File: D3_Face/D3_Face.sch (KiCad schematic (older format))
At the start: 31 parts, among them J1 Conn_01x05_Male, U1 MAX7219, U2 MAX7219, U3 MAX7219, U4 MAX7219, U5 MAX7219, U6 MAX7219

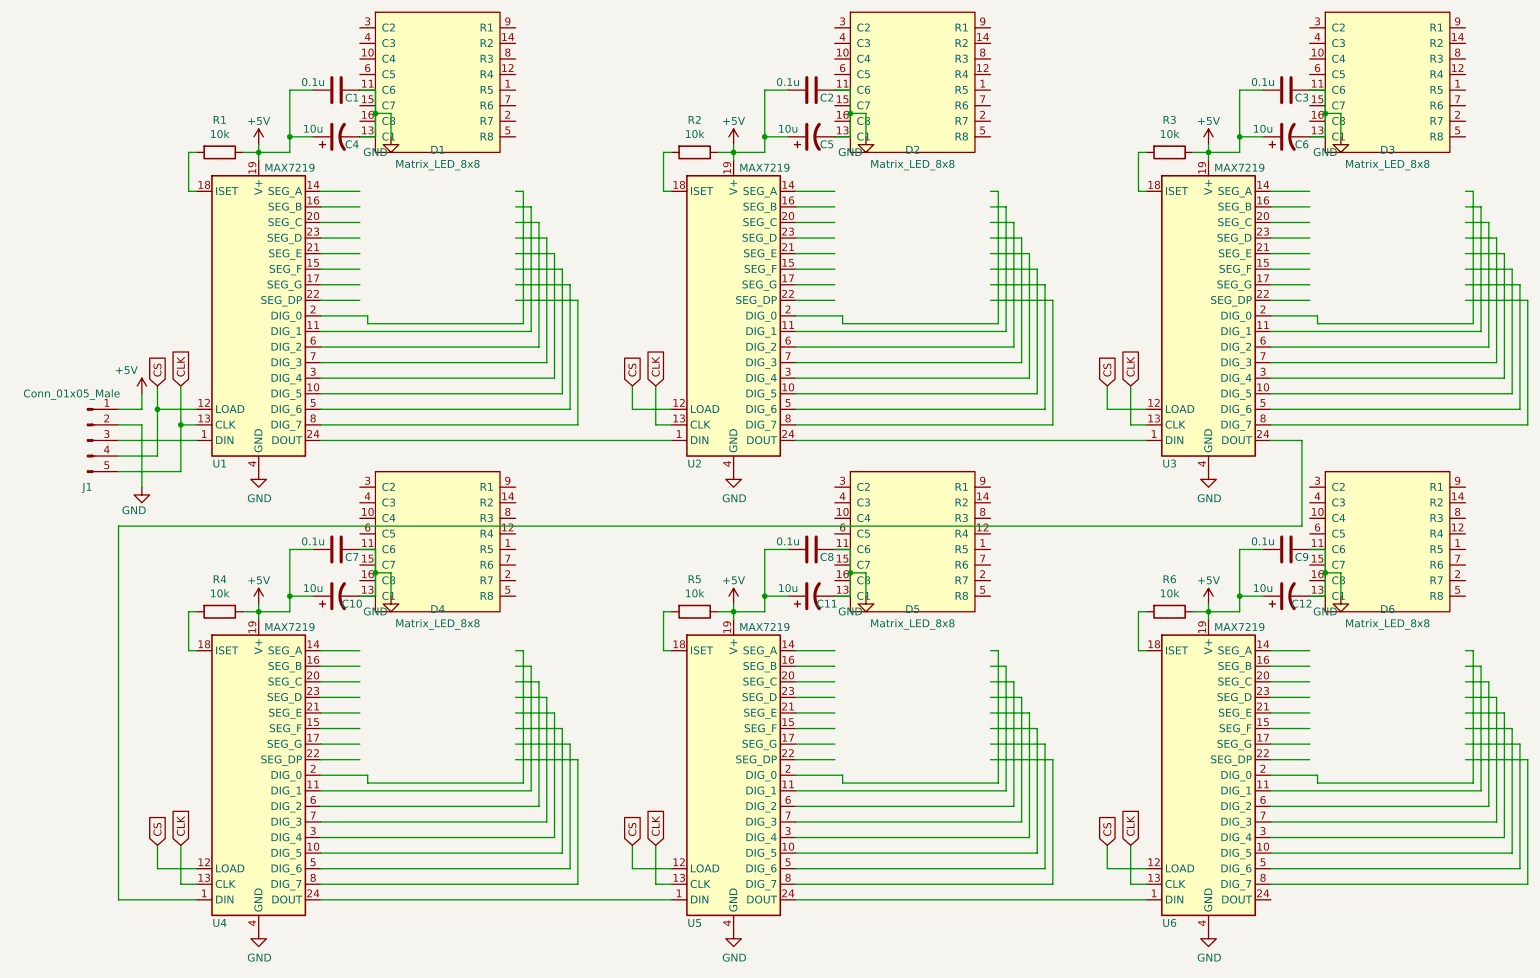
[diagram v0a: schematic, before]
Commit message: Create D3_Board
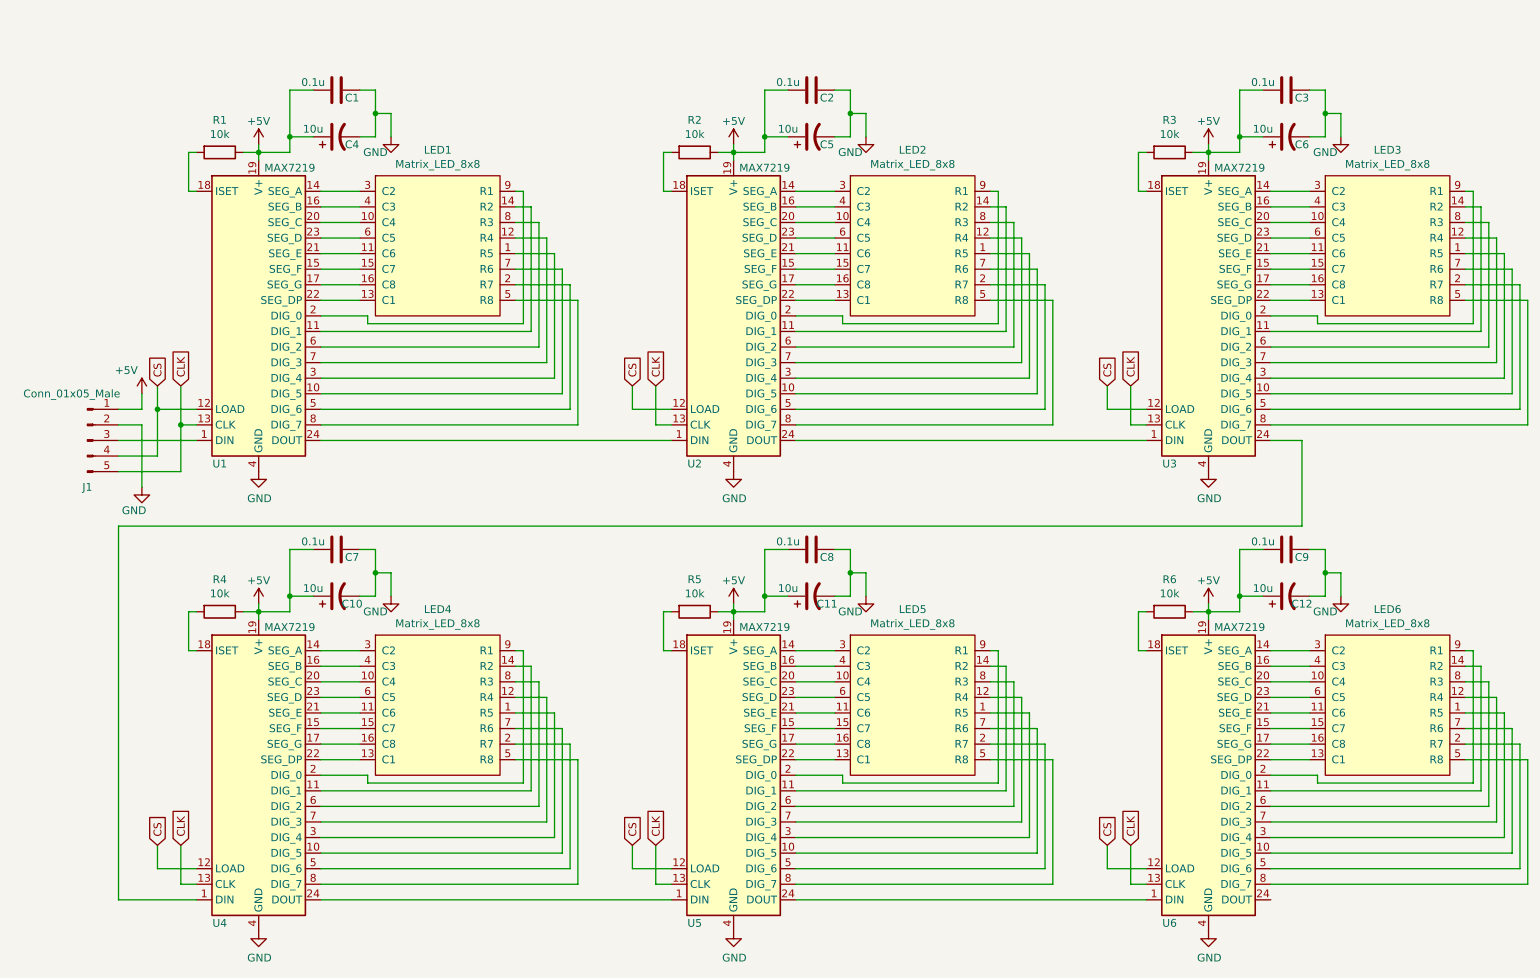
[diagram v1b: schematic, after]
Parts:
- removed D1, D2, D3, D4, D5, D6: Matrix_LED_8x8, D3_Face:Matrix_LED_8x8, symbol D3_Face:Matrix_LED_8x8
- added LED1, LED2, LED3, LED4, LED5, LED6: Matrix_LED_8x8, D3_Face:Matrix_LED_8x8, symbol D3_Face:Matrix_LED_8x8
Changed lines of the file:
@@
 	2650 1250 2650 1300
 $Comp
-L power:GND #PWR08
+L power:GND #PWR0101
 U 1 1 6006A3CE
 P 2650 3300
-F 0 "#PWR08" H 2650 3050 50  0001 C CNN
+F 0 "#PWR0101" H 2650 3050 50  0001 C CNN
 F 1 "GND" H 2655 3127 50  0000 C CNN
 F 2 "" H 2650 3300 50  0001 C CNN
@@
 Wire Wire Line
 	3050 2300 3350 2300
-$Comp
-L D3_Face:Matrix_LED_8x8 D1
-U 1 1 6005CBF2
-P 3800 1850
-F 0 "D1" H 3800 2465 50  0000 C CNN
-F 1 "Matrix_LED_8x8" H 3800 2374 50  0000 C CNN
-F 2 "D3_Face:Matrix_LED_8x8" H 3800 1300 50  0001 C CNN
-F 3 "" H 3800 1300 50  0001 C CNN
-	1    3800 1850
-	1    0    0    -1
-$EndComp
 Wire Wire Line
 	3050 1500 3300 1500
@@
 $EndComp
 $Comp
-L power:GND #PWR011
+L power:GND #PWR0102
 U 1 1 6007D025
 P 1900 3400
-F 0 "#PWR011" H 1900 3150 50  0001 C CNN
+F 0 "#PWR0102" H 1900 3150 50  0001 C CNN
 F 1 "GND" H 1850 3250 50  0000 C CNN
 F 2 "" H 1900 3400 50  0001 C CNN
@@
 $EndComp
 $Comp
-L power:+5V #PWR07
+L power:+5V #PWR0103
 U 1 1 6007BC2F
 P 1900 2800
-F 0 "#PWR07" H 1900 2650 50  0001 C CNN
+F 0 "#PWR0103" H 1900 2650 50  0001 C CNN
 F 1 "+5V" H 1800 2950 50  0000 C CNN
 F 2 "" H 1900 2800 50  0001 C CNN
@@
 	2150 2750 2150 3000
 $Comp
-L power:+5V #PWR04
+L power:+5V #PWR0104
 U 1 1 600A898F
 P 2650 1200
-F 0 "#PWR04" H 2650 1050 50  0001 C CNN
+F 0 "#PWR0104" H 2650 1050 50  0001 C CNN
 F 1 "+5V" H 2650 1350 50  0000 C CNN
 F 2 "" H 2650 1200 50  0001 C CNN
@@
 	3400 1150 3300 1150
 $Comp
-L power:GND #PWR01
+L power:GND #PWR0105
 U 1 1 600C792C
 P 3500 1150
-F 0 "#PWR01" H 3500 900 50  0001 C CNN
+F 0 "#PWR0105" H 3500 900 50  0001 C CNN
 F 1 "GND" H 3400 1050 50  0000 C CNN
 F 2 "" H 3500 1150 50  0001 C CNN
@@
 	5700 1250 5700 1300
 $Comp
-L power:GND #PWR09
+L power:GND #PWR0106
 U 1 1 60100772
 P 5700 3300
-F 0 "#PWR09" H 5700 3050 50  0001 C CNN
+F 0 "#PWR0106" H 5700 3050 50  0001 C CNN
 F 1 "GND" H 5705 3127 50  0000 C CNN
 F 2 "" H 5700 3300 50  0001 C CNN
@@
 Wire Wire Line
 	6100 2300 6400 2300
-$Comp
-L D3_Face:Matrix_LED_8x8 D2
-U 1 1 60100779
-P 6850 1850
-F 0 "D2" H 6850 2465 50  0000 C CNN
-F 1 "Matrix_LED_8x8" H 6850 2374 50  0000 C CNN
-F 2 "D3_Face:Matrix_LED_8x8" H 6850 1300 50  0001 C CNN
-F 3 "" H 6850 1300 50  0001 C CNN
-	1    6850 1850
-	1    0    0    -1
-$EndComp
 Wire Wire Line
 	6100 1500 6350 1500
@@
 	5200 2750 5200 3000
 $Comp
-L power:+5V #PWR05
+L power:+5V #PWR0107
 U 1 1 601007BE
 P 5700 1200
-F 0 "#PWR05" H 5700 1050 50  0001 C CNN
+F 0 "#PWR0107" H 5700 1050 50  0001 C CNN
 F 1 "+5V" H 5700 1350 50  0000 C CNN
 F 2 "" H 5700 1200 50  0001 C CNN
@@
 	6450 1150 6350 1150
 $Comp
-L power:GND #PWR02
+L power:GND #PWR0108
 U 1 1 601007CF
 P 6550 1150
-F 0 "#PWR02" H 6550 900 50  0001 C CNN
+F 0 "#PWR0108" H 6550 900 50  0001 C CNN
 F 1 "GND" H 6450 1050 50  0000 C CNN
 F 2 "" H 6550 1150 50  0001 C CNN
@@
 	8750 1250 8750 1300
 $Comp
-L power:GND #PWR010
+L power:GND #PWR0109
 U 1 1 6011D9CB
 P 8750 3300
-F 0 "#PWR010" H 8750 3050 50  0001 C CNN
+F 0 "#PWR0109" H 8750 3050 50  0001 C CNN
 F 1 "GND" H 8755 3127 50  0000 C CNN
 F 2 "" H 8750 3300 50  0001 C CNN
@@
 Wire Wire Line
 	9150 2300 9450 2300
-$Comp
-L D3_Face:Matrix_LED_8x8 D3
-U 1 1 6011D9D2
-P 9900 1850
-F 0 "D3" H 9900 2465 50  0000 C CNN
-F 1 "Matrix_LED_8x8" H 9900 2374 50  0000 C CNN
-F 2 "D3_Face:Matrix_LED_8x8" H 9900 1300 50  0001 C CNN
-F 3 "" H 9900 1300 50  0001 C CNN
-	1    9900 1850
-	1    0    0    -1
-$EndComp
 Wire Wire Line
 	9150 1500 9400 1500
@@
 	8250 2750 8250 3000
 $Comp
-L power:+5V #PWR06
+L power:+5V #PWR0110
 U 1 1 6011DA04
 P 8750 1200
-F 0 "#PWR06" H 8750 1050 50  0001 C CNN
+F 0 "#PWR0110" H 8750 1050 50  0001 C CNN
 F 1 "+5V" H 8750 1350 50  0000 C CNN
 F 2 "" H 8750 1200 50  0001 C CNN
@@
 	9500 1150 9400 1150
 $Comp
-L power:GND #PWR03
+L power:GND #PWR0111
 U 1 1 6011DA15
 P 9600 1150
-F 0 "#PWR03" H 9600 900 50  0001 C CNN
+F 0 "#PWR0111" H 9600 900 50  0001 C CNN
 F 1 "GND" H 9500 1050 50  0000 C CNN
 F 2 "" H 9600 1150 50  0001 C CNN
@@
 	2650 4200 2650 4250
 $Comp
-L power:GND #PWR018
+L power:GND #PWR0112
 U 1 1 60139852
 P 2650 6250
-F 0 "#PWR018" H 2650 6000 50  0001 C CNN
+F 0 "#PWR0112" H 2650 6000 50  0001 C CNN
 F 1 "GND" H 2655 6077 50  0000 C CNN
 F 2 "" H 2650 6250 50  0001 C CNN
@@
 Wire Wire Line
 	3050 5250 3350 5250
-$Comp
-L D3_Face:Matrix_LED_8x8 D4
-U 1 1 60139859
-P 3800 4800
-F 0 "D4" H 3800 5415 50  0000 C CNN
-F 1 "Matrix_LED_8x8" H 3800 5324 50  0000 C CNN
-F 2 "D3_Face:Matrix_LED_8x8" H 3800 4250 50  0001 C CNN
-F 3 "" H 3800 4250 50  0001 C CNN
-	1    3800 4800
-	1    0    0    -1
-$EndComp
 Wire Wire Line
 	3050 4450 3300 4450
@@
 	2150 5700 2150 5950
 $Comp
-L power:+5V #PWR015
+L power:+5V #PWR0113
 U 1 1 6013988D
 P 2650 4150
-F 0 "#PWR015" H 2650 4000 50  0001 C CNN
+F 0 "#PWR0113" H 2650 4000 50  0001 C CNN
 F 1 "+5V" H 2650 4300 50  0000 C CNN
 F 2 "" H 2650 4150 50  0001 C CNN
@@
 	3400 4100 3300 4100
 $Comp
-L power:GND #PWR012
+L power:GND #PWR0114
 U 1 1 6013989E
 P 3500 4100
-F 0 "#PWR012" H 3500 3850 50  0001 C CNN
+F 0 "#PWR0114" H 3500 3850 50  0001 C CNN
 F 1 "GND" H 3400 4000 50  0000 C CNN
 F 2 "" H 3500 4100 50  0001 C CNN
@@
 	5700 4200 5700 4250
 $Comp
-L power:GND #PWR019
+L power:GND #PWR0115
 U 1 1 601398C0
 P 5700 6250
-F 0 "#PWR019" H 5700 6000 50  0001 C CNN
+F 0 "#PWR0115" H 5700 6000 50  0001 C CNN
 F 1 "GND" H 5705 6077 50  0000 C CNN
 F 2 "" H 5700 6250 50  0001 C CNN
@@
 	5200 5700 5200 5950
 $Comp
-L power:+5V #PWR016
+L power:+5V #PWR0116
 U 1 1 601398F9
 P 5700 4150
-F 0 "#PWR016" H 5700 4000 50  0001 C CNN
+F 0 "#PWR0116" H 5700 4000 50  0001 C CNN
 F 1 "+5V" H 5700 4300 50  0000 C CNN
 F 2 "" H 5700 4150 50  0001 C CNN
@@
 	6450 4100 6350 4100
 $Comp
-L power:GND #PWR013
+L power:GND #PWR0117
 U 1 1 6013990A
 P 6550 4100
-F 0 "#PWR013" H 6550 3850 50  0001 C CNN
+F 0 "#PWR0117" H 6550 3850 50  0001 C CNN
 F 1 "GND" H 6450 4000 50  0000 C CNN
 F 2 "" H 6550 4100 50  0001 C CNN
@@
 	8750 4200 8750 4250
 $Comp
-L power:GND #PWR020
+L power:GND #PWR0118
 U 1 1 6013992D
 P 8750 6250
-F 0 "#PWR020" H 8750 6000 50  0001 C CNN
+F 0 "#PWR0118" H 8750 6000 50  0001 C CNN
 F 1 "GND" H 8755 6077 50  0000 C CNN
 F 2 "" H 8750 6250 50  0001 C CNN
@@
 Wire Wire Line
 	9150 5250 9450 5250
-$Comp
-L D3_Face:Matrix_LED_8x8 D6
-U 1 1 60139934
-P 9900 4800
-F 0 "D6" H 9900 5415 50  0000 C CNN
-F 1 "Matrix_LED_8x8" H 9900 5324 50  0000 C CNN
-F 2 "D3_Face:Matrix_LED_8x8" H 9900 4250 50  0001 C CNN
-F 3 "" H 9900 4250 50  0001 C CNN
-	1    9900 4800
-	1    0    0    -1
-$EndComp
 Wire Wire Line
 	9150 4450 9400 4450
@@
 	8250 5700 8250 5950
 $Comp
-L power:+5V #PWR017
+L power:+5V #PWR0119
 U 1 1 60139966
 P 8750 4150
-F 0 "#PWR017" H 8750 4000 50  0001 C CNN
+F 0 "#PWR0119" H 8750 4000 50  0001 C CNN
 F 1 "+5V" H 8750 4300 50  0000 C CNN
 F 2 "" H 8750 4150 50  0001 C CNN
@@
 	9500 4100 9400 4100
 $Comp
-L power:GND #PWR014
+L power:GND #PWR0120
 U 1 1 60139977
 P 9600 4100
-F 0 "#PWR014" H 9600 3850 50  0001 C CNN
+F 0 "#PWR0120" H 9600 3850 50  0001 C CNN
 F 1 "GND" H 9500 4000 50  0000 C CNN
 F 2 "" H 9600 4100 50  0001 C CNN
@@
 	6400 5300 7400 5300
 $Comp
-L D3_Face:Matrix_LED_8x8 D5
-U 1 1 601398C7
-P 6850 4800
-F 0 "D5" H 6850 5415 50  0000 C CNN
-F 1 "Matrix_LED_8x8" H 6850 5324 50  0000 C CNN
-F 2 "D3_Face:Matrix_LED_8x8" H 6850 4250 50  0001 C CNN
-F 3 "" H 6850 4250 50  0001 C CNN
-	1    6850 4800
-	1    0    0    -1
-$EndComp
+L D3_Face:Matrix_LED_8x8 LED2
+U 1 1 60217BCD
+P 6850 2900
+F 0 "LED2" H 6850 4565 50  0000 C CNN
+F 1 "Matrix_LED_8x8" H 6850 4474 50  0000 C CNN
+F 2 "D3_Face:Matrix_LED_8x8" H 6850 3300 50  0001 C CNN
+F 3 "" H 6850 3400 50  0001 C CNN
+	1    6850 2900
+	1    0    0    -1
+$EndComp
+$Comp
+L D3_Face:Matrix_LED_8x8 LED3
+U 1 1 60219CA7
+P 9900 2900
+F 0 "LED3" H 9900 4565 50  0000 C CNN
+F 1 "Matrix_LED_8x8" H 9900 4474 50  0000 C CNN
+F 2 "D3_Face:Matrix_LED_8x8" H 9900 3300 50  0001 C CNN
+F 3 "" H 9900 3400 50  0001 C CNN
+	1    9900 2900
+	1    0    0    -1
+$EndComp
+$Comp
+L D3_Face:Matrix_LED_8x8 LED6
+U 1 1 6021CE0E
+P 9900 5850
+F 0 "LED6" H 9900 7515 50  0000 C CNN
+F 1 "Matrix_LED_8x8" H 9900 7424 50  0000 C CNN
+F 2 "D3_Face:Matrix_LED_8x8" H 9900 6250 50  0001 C CNN
+F 3 "" H 9900 6350 50  0001 C CNN
+	1    9900 5850
+	1    0    0    -1
+$EndComp
+$Comp
+L D3_Face:Matrix_LED_8x8 LED5
+U 1 1 6021F0CD
+P 6850 5850
+F 0 "LED5" H 6850 7515 50  0000 C CNN
+F 1 "Matrix_LED_8x8" H 6850 7424 50  0000 C CNN
+F 2 "D3_Face:Matrix_LED_8x8" H 6850 6250 50  0001 C CNN
+F 3 "" H 6850 6350 50  0001 C CNN
+	1    6850 5850
+	1    0    0    -1
+$EndComp
+$Comp
+L D3_Face:Matrix_LED_8x8 LED4
+U 1 1 60220F3B
+P 3800 5850
+F 0 "LED4" H 3800 7515 50  0000 C CNN
+F 1 "Matrix_LED_8x8" H 3800 7424 50  0000 C CNN
+F 2 "D3_Face:Matrix_LED_8x8" H 3800 6250 50  0001 C CNN
+F 3 "" H 3800 6350 50  0001 C CNN
+	1    3800 5850
+	1    0    0    -1
+$EndComp
+$Comp
+L D3_Face:Matrix_LED_8x8 LED1
+U 1 1 60203125
+P 3800 2900
+F 0 "LED1" H 3800 4565 50  0000 C CNN
+F 1 "Matrix_LED_8x8" H 3800 4474 50  0000 C CNN
+F 2 "D3_Face:Matrix_LED_8x8" H 3800 3300 50  0001 C CNN
+F 3 "" H 3800 3400 50  0001 C CNN
+	1    3800 2900
+	1    0    0    -1
+$EndComp
